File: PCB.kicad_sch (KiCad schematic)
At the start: 2 parts

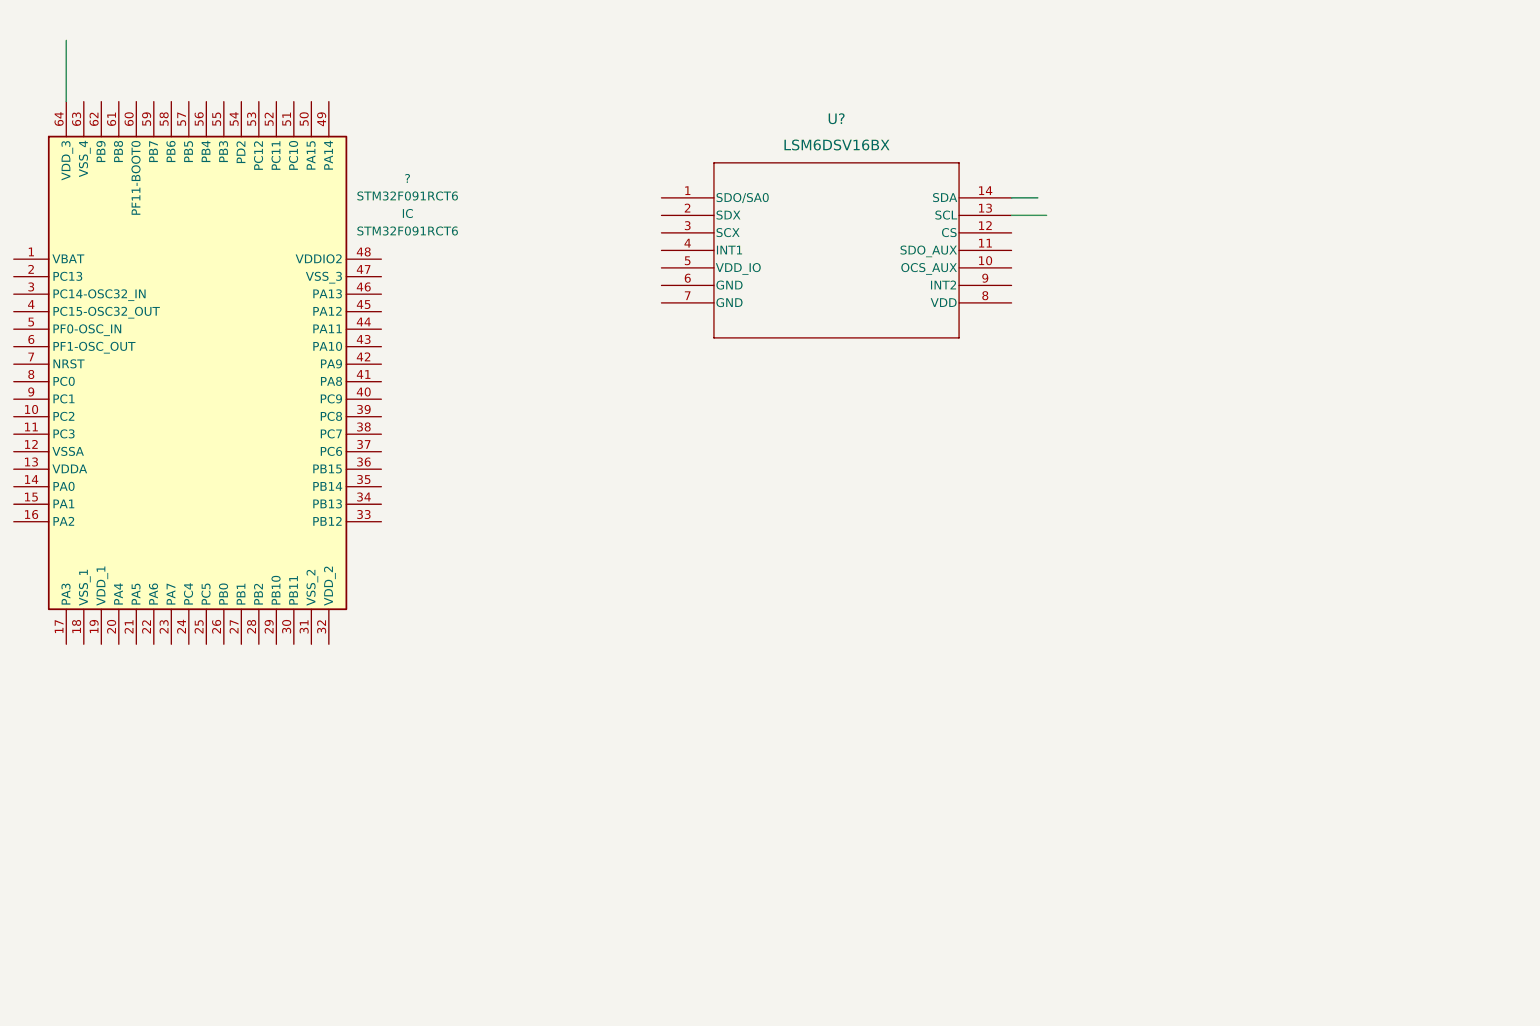
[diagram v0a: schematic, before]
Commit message: new stuff
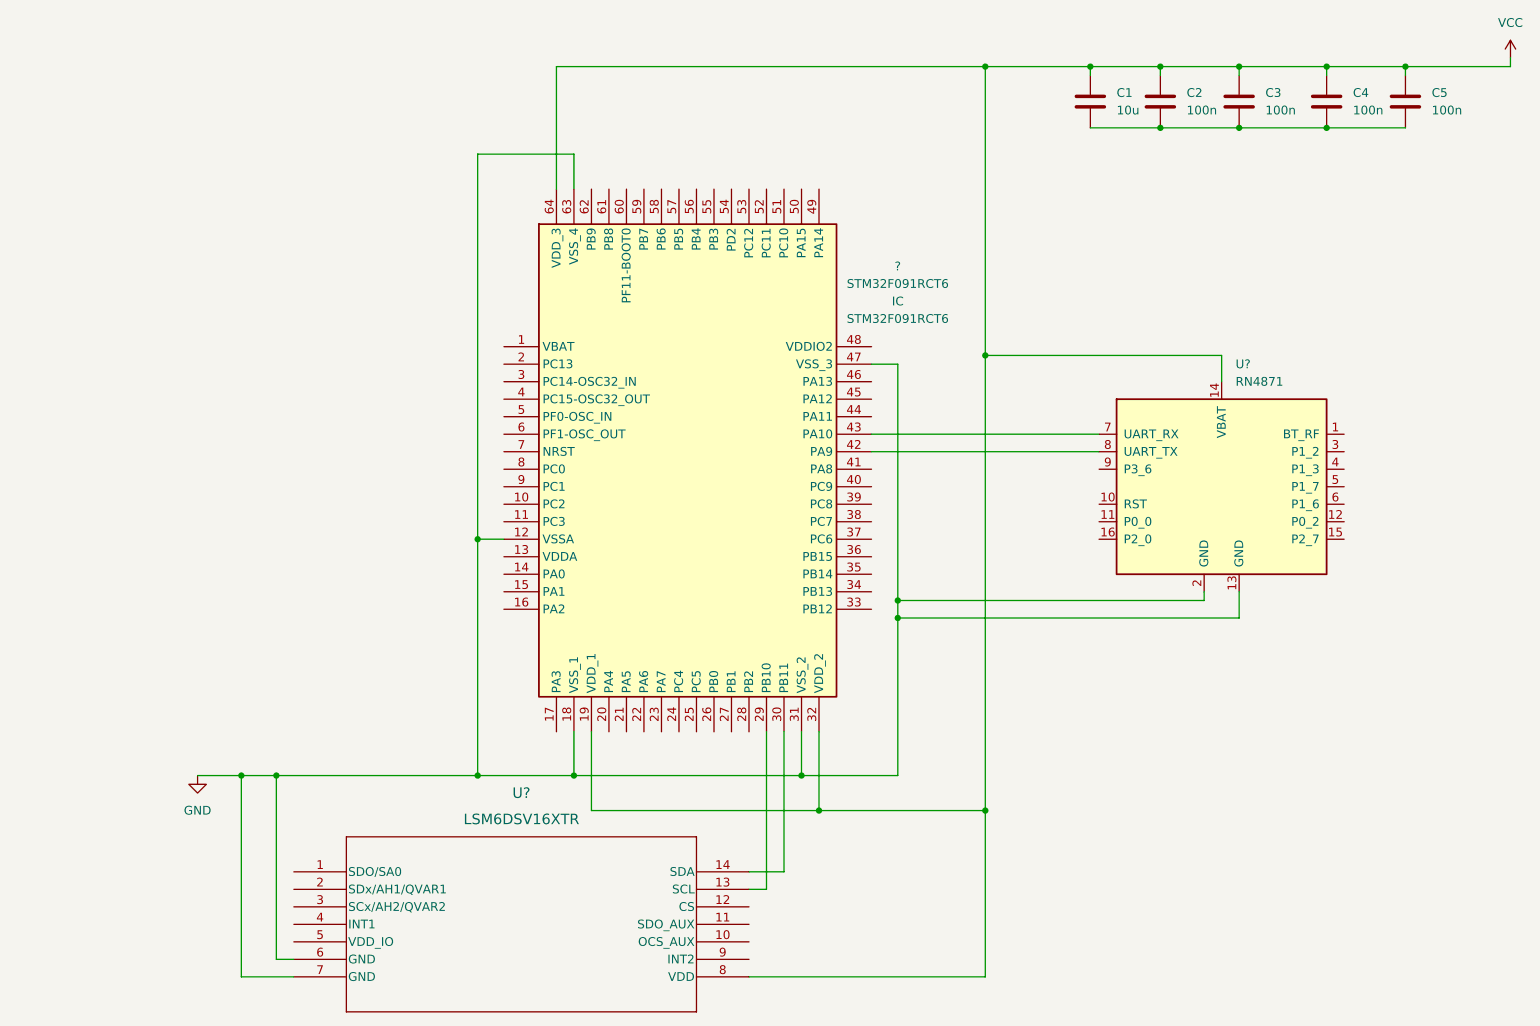
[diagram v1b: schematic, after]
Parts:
- removed U?: LSM6DSV16BX, LGA14L_2P59X3P1X0P5_STM, symbol 2023-09-13_16-10-09:LSM6DSV16BX
- added C1: 10u, symbol Device:C
- added C2, C3, C4, C5: 100n, symbol Device:C
- added U?: RN4871, RF_Module:Microchip_RN4871, symbol RF_Bluetooth:RN4871
- added U?: LSM6DSV16XTR, LGA14L_LSM6_STM, symbol LSM6DSV16XTR:LSM6DSV16XTR
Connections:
- net GND: now reaches ?.12 (VSSA)
- net GND: now also ?.18 (VSS_1), ?.31 (VSS_2), ?.47 (VSS_3), ?.63 (VSS_4), U?.13 (GND), U?.2 (GND), U?.6 (GND), U?.7 (GND)
- net VCC: now reaches ?.19 (VDD_1)
- net VCC: now also ?.32 (VDD_2), ?.64 (VDD_3), C1.1, C2.1, C3.1, C4.1, C5.1, U?.14 (VBAT), U?.8 (VDD)
- net at ?.29 (PB10): now also U?.13 (SCL)
- net at ?.30 (PB11): now also U?.14 (SDA)
- net at ?.42 (PA9): now also U?.8 (UART_TX)
- net at ?.43 (PA10): now also U?.7 (UART_RX)
- new net: C1.2, C2.2, C3.2, C4.2, C5.2
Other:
- moved on the sheet: ?
